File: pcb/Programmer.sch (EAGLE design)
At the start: 5 parts, among them J1 MINI-USB-JACK, U1 FT232HQ, U2 SN74AVCH4T245RSVR, X1 SIT8021

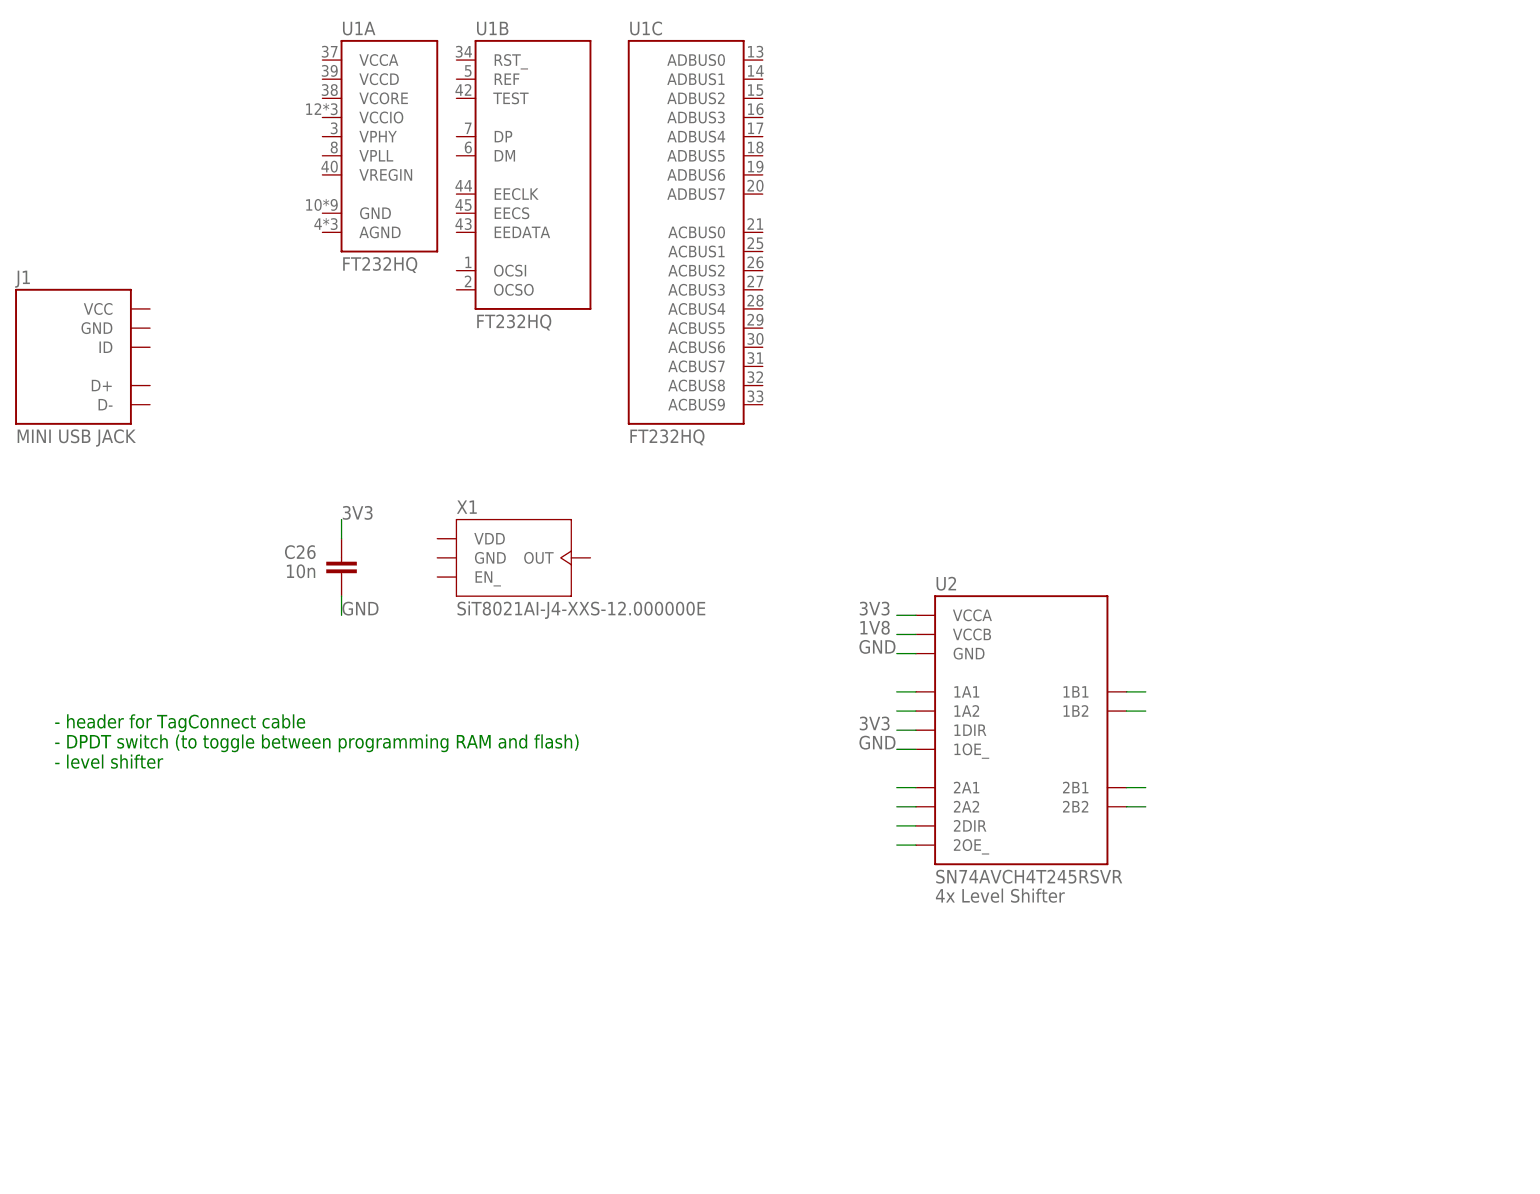
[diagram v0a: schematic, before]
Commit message: Progress creating programmer board
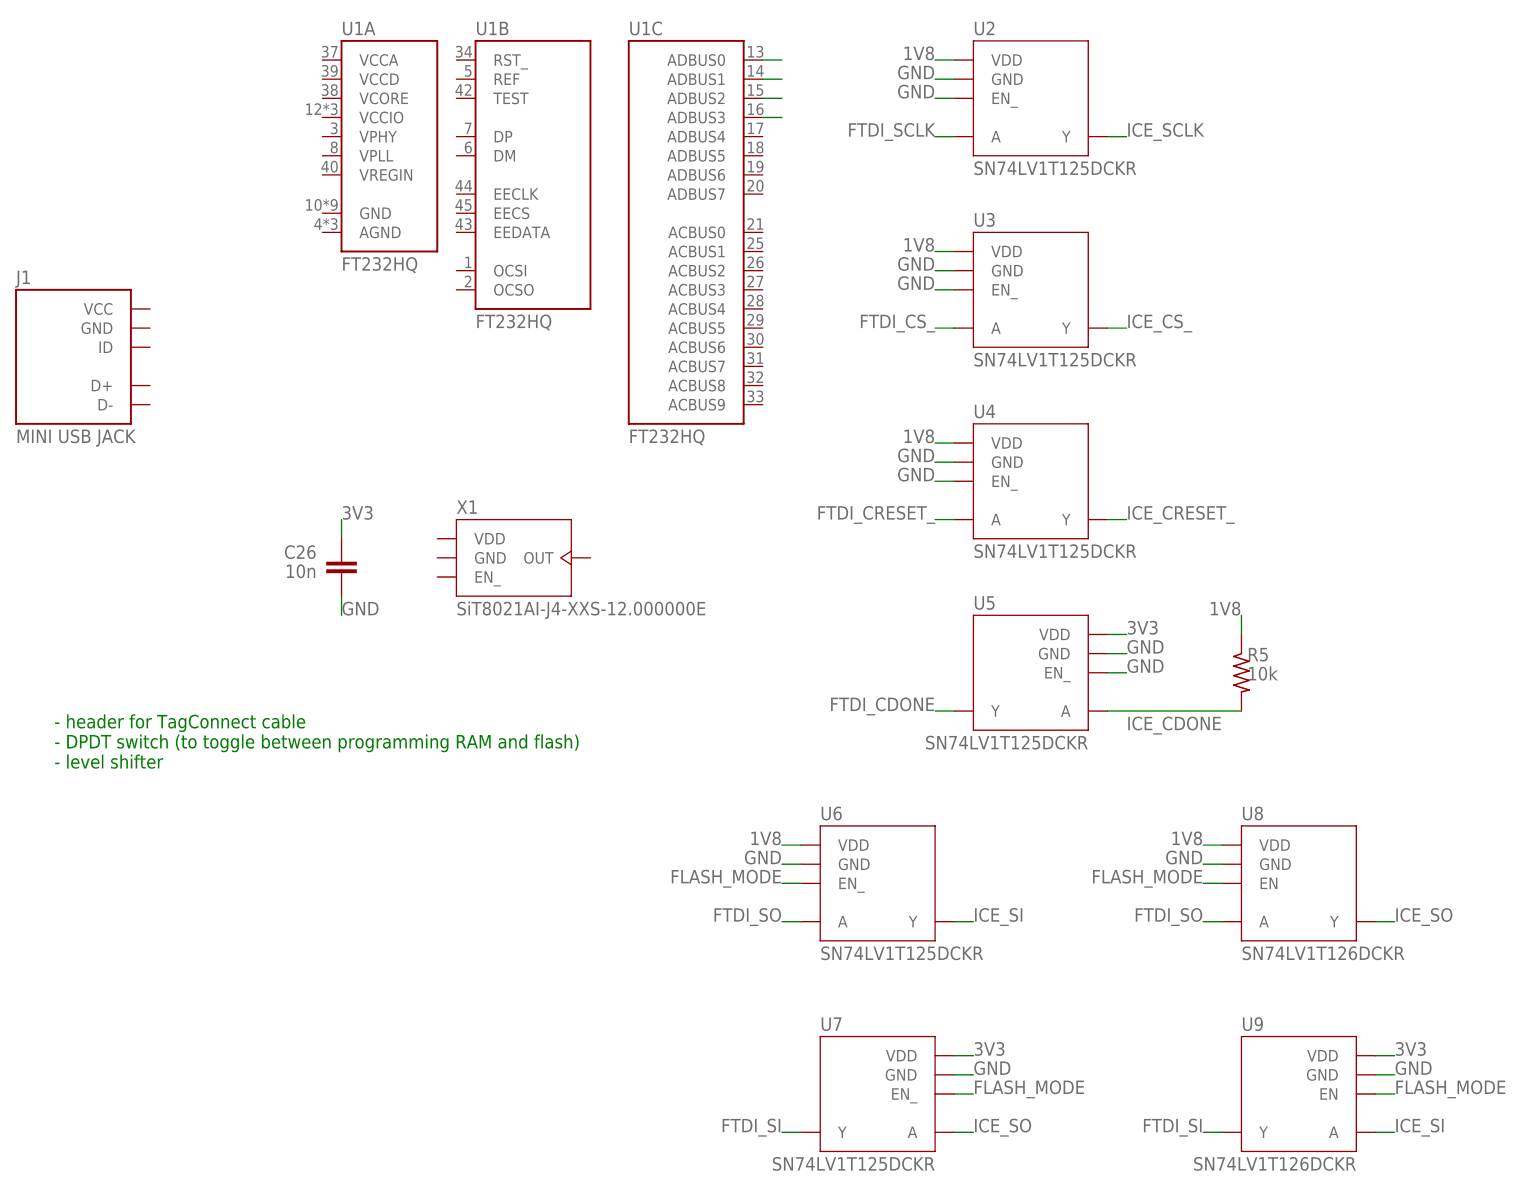
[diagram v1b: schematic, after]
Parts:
- added R5: 10k, EagleLibrary:RESISTOR0402
- added U3, U4, U5, U6, U7: SN74LV1T125DCKR, EagleLibrary:SN74LV1T125DCKR
- added U8, U9: SN74LV1T126DCKR, EagleLibrary:SN74LV1T126DCKR
- U2: value SN74AVCH4T245RSVR -> SN74LV1T125DCKR; device EagleLibrary:SN74AVCH4T245RSVR -> EagleLibrary:SN74LV1T125DCKR
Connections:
- removed net N$10: U2.2OE_
- removed net N$12: U2.2DIR
- removed net N$5: U2.2A1
- removed net N$6: U2.2A2
- removed net N$7: U2.2B1
- removed net N$8: U2.2B2
- new net FLASH_MODE: U6.EN_, U7.EN_, U8.EN, U9.EN
- new net FTDI_CDONE: U5.Y
- new net FTDI_CRESET_: U4.A
- new net FTDI_CS_: U3.A
- new net FTDI_SCLK: U2.A
- new net FTDI_SI: U7.Y, U9.Y
- new net FTDI_SO: U6.A, U8.A
- new net ICE_CDONE: R5.2, U5.A
- new net ICE_CRESET_: U4.Y
- new net ICE_CS_: U3.Y
- new net ICE_SCLK: U2.Y
- new net ICE_SI: U6.Y, U9.A
- new net ICE_SO: U7.A, U8.Y
- net 1V8: now also R5.1, U2.VDD, U3.VDD, U4.VDD, U6.VDD, U8.VDD; no longer U2.VCCB
- net 3V3: now also U5.VDD, U7.VDD, U9.VDD; no longer U2.1DIR, U2.VCCA
- net GND: now also U2.EN_, U3.EN_, U3.GND, U4.EN_, U4.GND, U5.EN_, U5.GND, U6.GND, U7.GND, U8.GND, U9.GND; no longer U2.1OE_
- net N$1: now also U1C.ADBUS0; no longer U2.1A1
- net N$2: now also U1C.ADBUS1; no longer U2.1A2
- net N$3: now also U1C.ADBUS2; no longer U2.1B1
- net N$4: now also U1C.ADBUS3; no longer U2.1B2
